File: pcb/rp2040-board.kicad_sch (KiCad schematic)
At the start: 35 parts, among them J2 GPIO, J3 ELRS, J4 OLED, J5 SWD, SW1 TS-1187A-B-A-B, SW2 RotaryEncoder_Switch, SW3 TS-1187A-B-A-B, U1 W25Q128JVS, U3 RP2040, Y1 12MHz

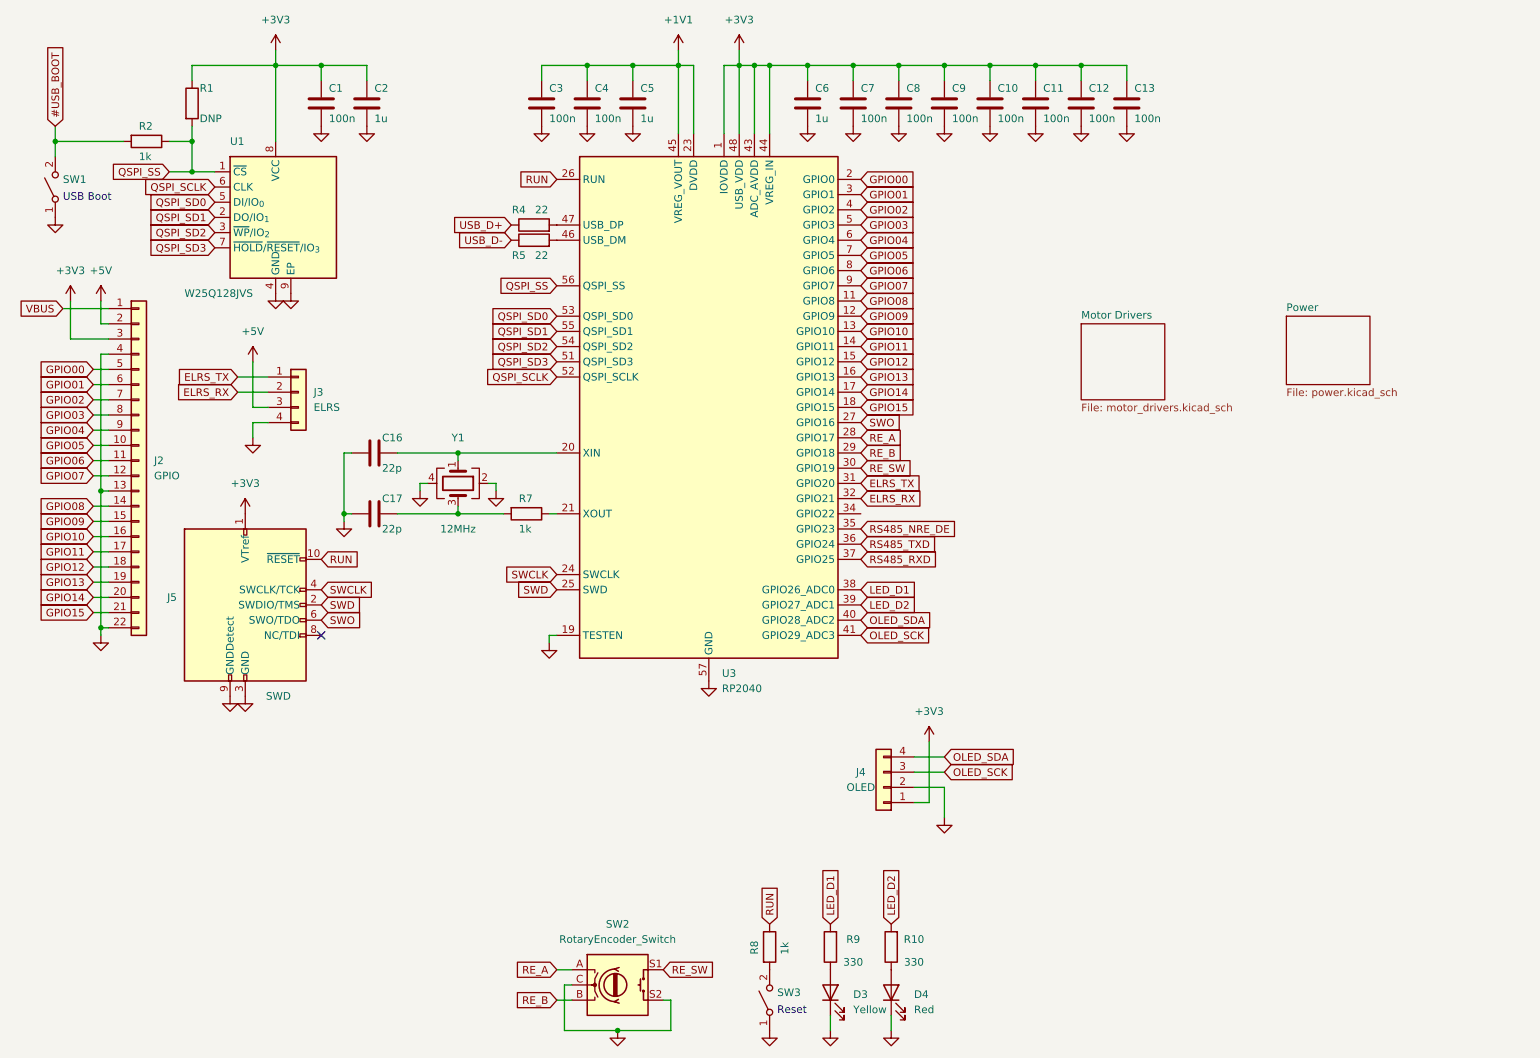
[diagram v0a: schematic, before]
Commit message: WIP on the motor driver board
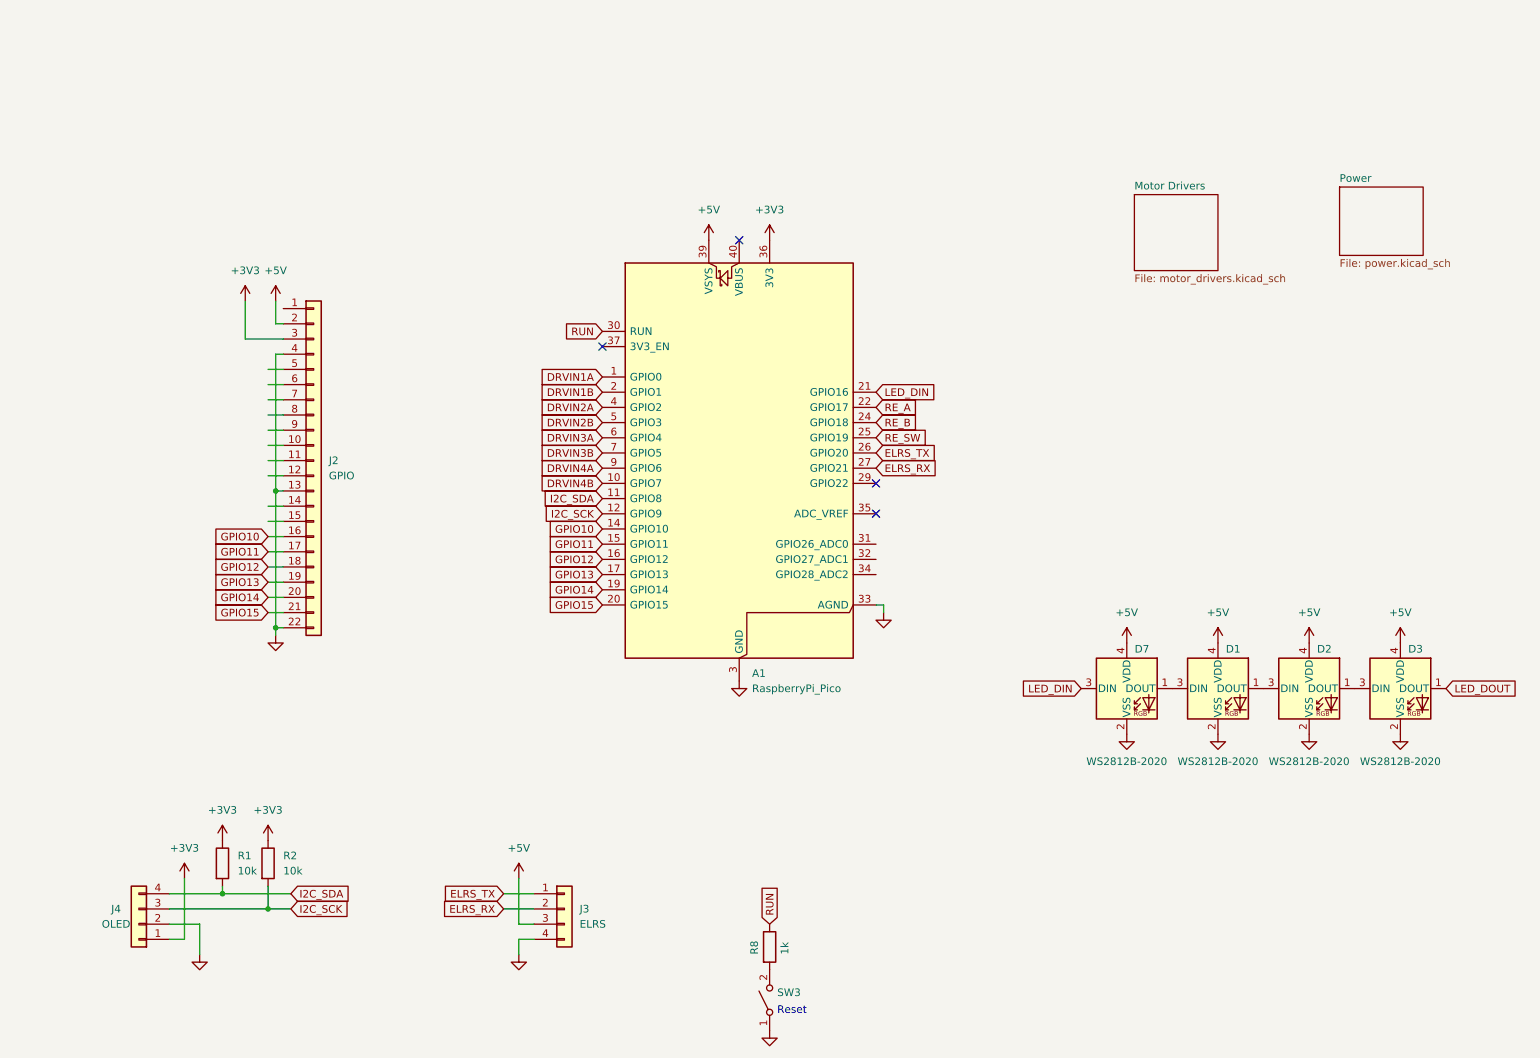
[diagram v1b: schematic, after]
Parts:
- removed C1, C10, C11, C12, C13, C3, C4, C7, C8, C9: 100n, Capacitor_SMD:C_0402_1005Metric, symbol Device:C
- removed C16, C17: 22p, Capacitor_SMD:C_0402_1005Metric, symbol Device:C
- removed C2, C5, C6: 1u, Capacitor_SMD:C_0402_1005Metric, symbol Device:C
- removed D3: Yellow, LED_SMD:LED_0603_1608Metric, symbol Device:LED
- removed D4: Red, LED_SMD:LED_0603_1608Metric, symbol Device:LED
- removed J5: SWD, Connector_PinHeader_1.27mm:PinHeader_2x05_P1.27mm_Vertical_SMD, symbol Connector:Conn_ARM_JTAG_SWD_10
- removed R10, R9: 330, Resistor_SMD:R_0402_1005Metric, symbol Device:R
- removed R4, R5: 22, Resistor_SMD:R_0402_1005Metric, symbol Device:R
- removed R7: 1k, Resistor_SMD:R_0402_1005Metric, symbol Device:R
- removed SW1: TS-1187A-B-A-B, Button_Switch_SMD:SW_Push_1P1T_XKB_TS-1187A, symbol Switch:SW_SPST
- removed SW2: RotaryEncoder_Switch, Rotary_Encoder:RotaryEncoder_Bourns_Vertical_PEC12R-3x17F-Sxxxx, symbol Device:RotaryEncoder_Switch
- removed U1: W25Q128JVS, Package_SON:WSON-8-1EP_6x5mm_P1.27mm_EP3.4x4.3mm, symbol Memory_Flash:W25Q32JVZP
- removed U3: RP2040, Package_DFN_QFN:QFN-56-1EP_7x7mm_P0.4mm_EP3.2x3.2mm, symbol MCU_RaspberryPi:RP2040
- removed Y1: 12MHz, Crystal:Crystal_SMD_3225-4Pin_3.2x2.5mm, symbol Device:Crystal_GND24
- added A1: RaspberryPi_Pico, Module:RaspberryPi_Pico_Common_Unspecified, symbol MCU_Module:RaspberryPi_Pico
- added D1, D2, D3, D7: WS2812B-2020, LED_SMD:LED_WS2812B-2020_PLCC4_2.0x2.0mm, symbol LED:WS2812B-2020
- R1: value DNP -> 10k; JLCPCB BOM false -> (none); LCSC Part (none) -> C25744
- R2: value 1k -> 10k; LCSC Part C11702 -> C25744
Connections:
- net OLED_SCK is gone; now on net I2C_SCK: J4.3 (Pin_3)
- net +3V3: now also R2.1, A1.36 (3V3)
- net +5V: now also A1.39 (VSYS), D1.4 (VDD), D2.4 (VDD), D3.4 (VDD), D7.4 (VDD)
- net ELRS_RX: now also A1.27 (GPIO21)
- net ELRS_TX: now also A1.26 (GPIO20)
- net GND: now also A1.13 (GND), A1.18 (GND), A1.23 (GND), A1.28 (GND), A1.3 (GND), A1.33 (AGND), A1.38 (GND), A1.8 (GND), D1.2 (VSS), D2.2 (VSS), D3.2 (VSS), D7.2 (VSS)
- net GPIO10: now also A1.14 (GPIO10)
- net GPIO11: now also A1.15 (GPIO11)
- net GPIO12: now also A1.16 (GPIO12)
- net GPIO13: now also A1.17 (GPIO13)
- net GPIO14: now also A1.19 (GPIO14)
- net GPIO15: now also A1.20 (GPIO15)
- net RE_A: now also A1.22 (GPIO17)
- net RE_B: now also A1.24 (GPIO18)
- net RE_SW: now also A1.25 (GPIO19)
- net RUN: now also A1.30 (RUN)
- net #USB_BOOT renamed I2C_SCK
- net I2C_SCK: now also A1.12 (GPIO9)
- net GPIO00: no longer names the net of J2.5 (Pin_5)
- net GPIO01: no longer names the net of J2.6 (Pin_6)
- net GPIO02: no longer names the net of J2.7 (Pin_7)
- net GPIO03: no longer names the net of J2.8 (Pin_8)
- net GPIO04: no longer names the net of J2.9 (Pin_9)
- net GPIO05: no longer names the net of J2.10 (Pin_10)
- net GPIO06: no longer names the net of J2.11 (Pin_11)
- net GPIO07: no longer names the net of J2.12 (Pin_12)
- net GPIO08: no longer names the net of J2.14 (Pin_14)
- net GPIO09: no longer names the net of J2.15 (Pin_15)
- net OLED_SDA renamed I2C_SDA
- net I2C_SDA: now also R1.2, A1.11 (GPIO8)
- removed net QSPI_SS: R1.2, R2.1
- net VBUS: no longer names the net of J2.1 (Pin_1)
- new net: D2.1 (DOUT), D3.3 (DIN)
- new net: D1.1 (DOUT), D2.3 (DIN)
- new net: D1.3 (DIN), D7.1 (DOUT)
- new net DRVIN1A: A1.1 (GPIO0)
- new net DRVIN1B: A1.2 (GPIO1)
- new net DRVIN2A: A1.4 (GPIO2)
- new net DRVIN2B: A1.5 (GPIO3)
- new net DRVIN3A: A1.6 (GPIO4)
- new net DRVIN3B: A1.7 (GPIO5)
- new net DRVIN4A: A1.9 (GPIO6)
- new net DRVIN4B: A1.10 (GPIO7)
- new net LED_DIN: A1.21 (GPIO16), D7.3 (DIN)
- new net LED_DOUT: D3.1 (DOUT)
- no-connect marks 1 -> 4
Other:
- note removed: "USB Boot"
- moved on the sheet: J2, J3, J4

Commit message: wip on pcb
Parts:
- A1: footprint Module:RaspberryPi_Pico_Common_Unspecified -> Module:RaspberryPi_Pico_Common_SMD
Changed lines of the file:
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@@
 			)
 		)
-		(property "Footprint" "Module:RaspberryPi_Pico_Common_Unspecified"
+		(property "Footprint" "Module:RaspberryPi_Pico_Common_SMD"
 			(at 134.62 142.24 0)
 			(effects
